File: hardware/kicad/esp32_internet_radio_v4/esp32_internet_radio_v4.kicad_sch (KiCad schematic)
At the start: 17 parts, among them J1 ENCODER, J2 RGB LED, J3 ST7789, J4 extend, J5 POWER_IN_5V, J6 PCM5102, J7 TFT_SPI, P1 Power, P2 Analog, P3 Digital, P4 Digital, P5 CONN_01X01, P6 CONN_01X01, P7 CONN_01X01, P8 CONN_01X01

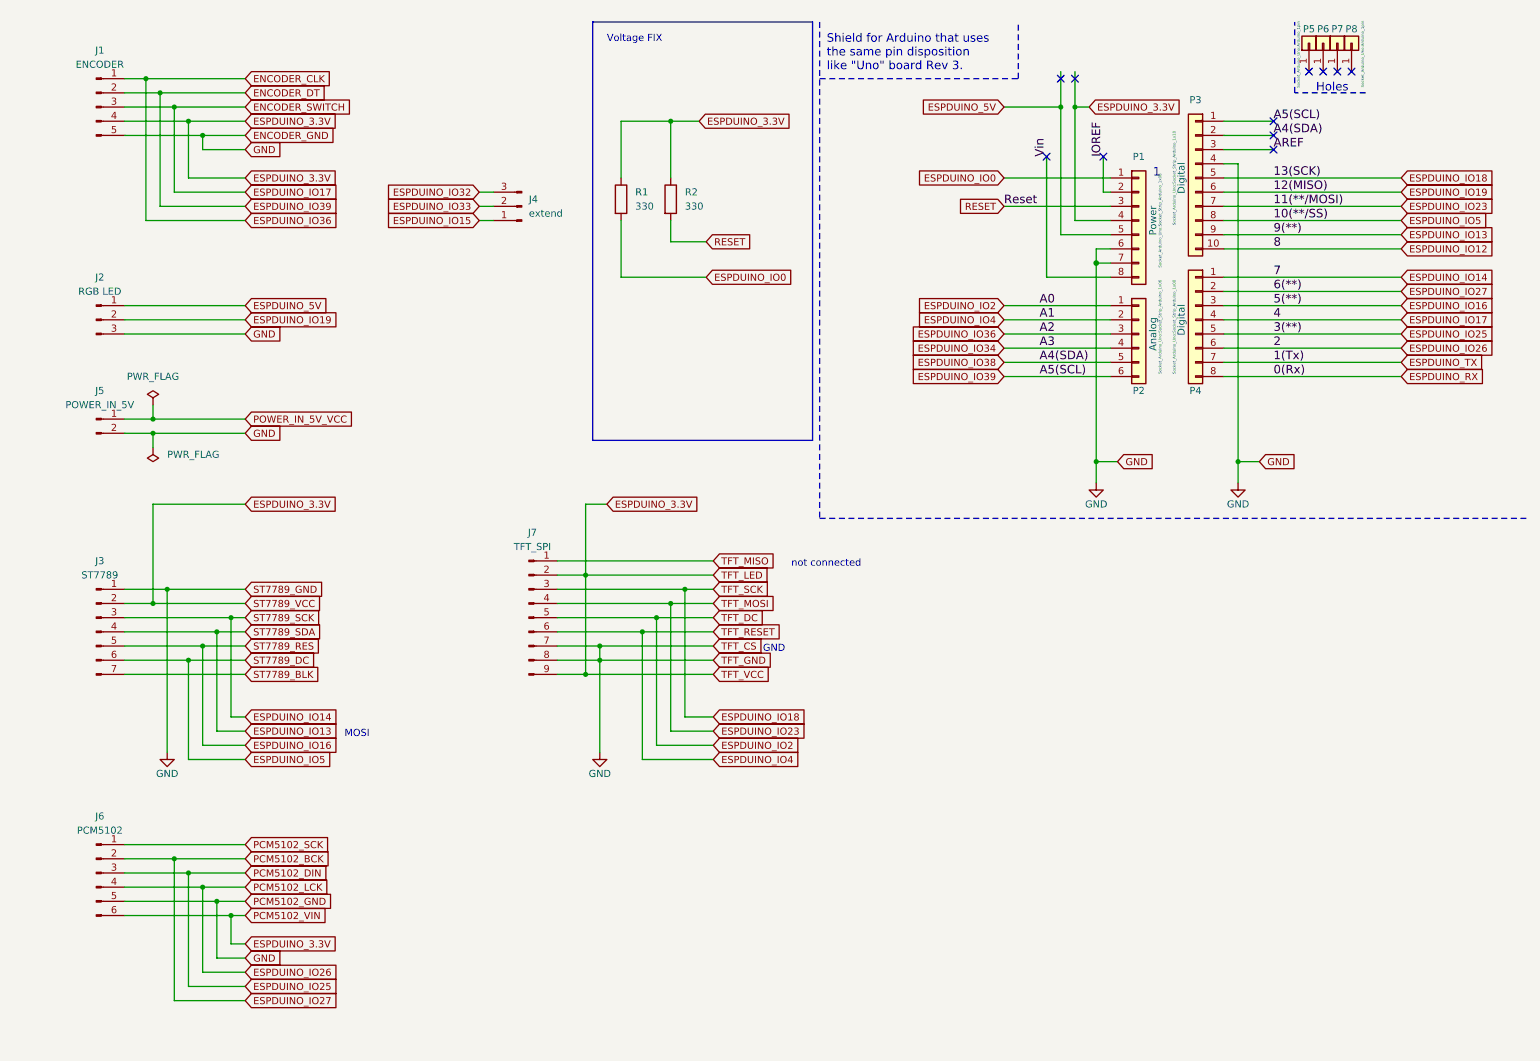
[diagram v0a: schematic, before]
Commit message: update schematics
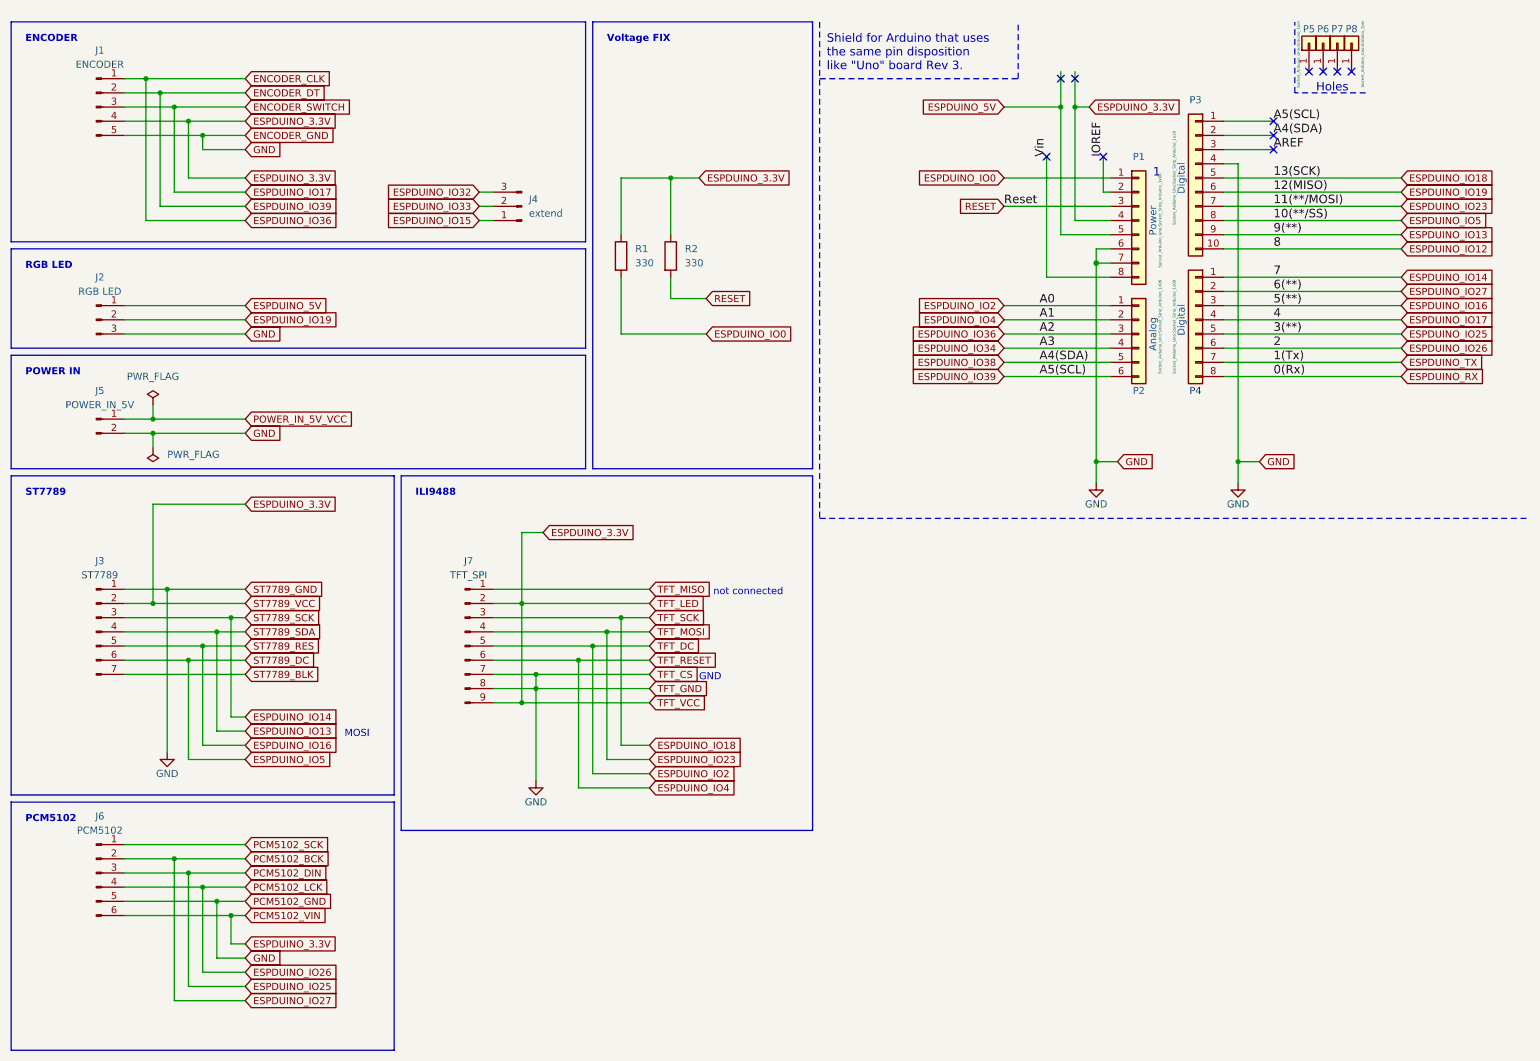
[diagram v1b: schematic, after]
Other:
- note added: "ENCODER"
- note added: "ILI9488"
- note added: "PCM5102"
- note added: "POWER IN"
- note added: "RGB LED"
- note added: "ST7789"
- moved on the sheet: J7, R1, R2
